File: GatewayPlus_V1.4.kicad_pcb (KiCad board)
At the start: 2 copper layers, 100 x 60 mm, 274 parts, among them IC1 MP1584EN, IC2 MP1584EN, J1 SWD_LOG, J10 USB_OTG, J11 USB_WIFI, J2 LTDC_LCD_FPC_40p, J3 Micro_SD_Card, J4 ESP Anten, J5 LoRa_Anten, J6 HR911105A, J7 RS485, J8 Conn_Jack-DC, J9 AudioJack, Q1 BC847, SW1 SW_Push, SW2 ESP_RESET, SW3 ESP_BOOT, U1 STM32F429IGTx, U10 USBLC6-2SC6, U11 USBLC6-2SC6, U2 IS42S16400J - HY57V641620E, U3 ESP32-C3, U4 W25Q32JVSS, U5 SX1278, U6 MASWSS0192, U7 LAN8720A, U8 MAX485E, U9 ES8388, Y1 25MHz, Y2 40MHz, Y3 32MHz, Y4 25MHz, Y5 32.768KHz

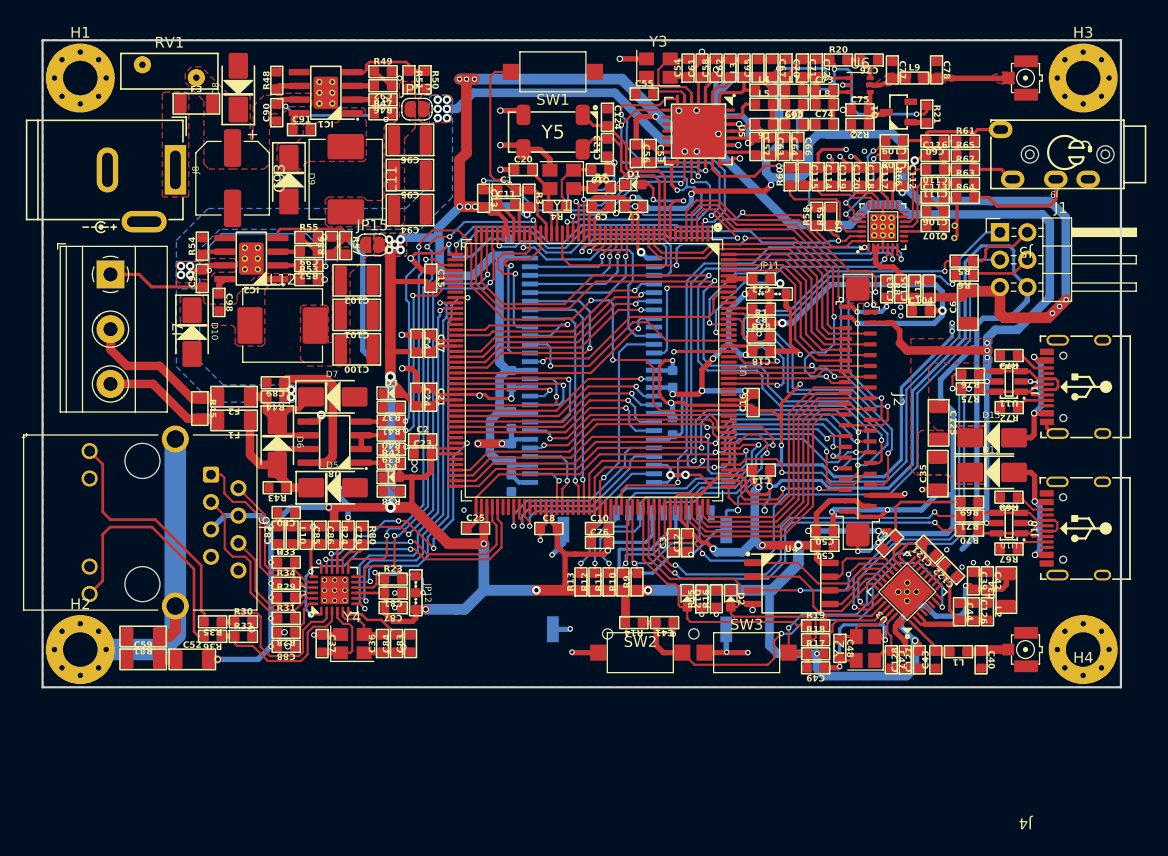
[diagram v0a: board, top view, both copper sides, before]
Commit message: Fix some bug.
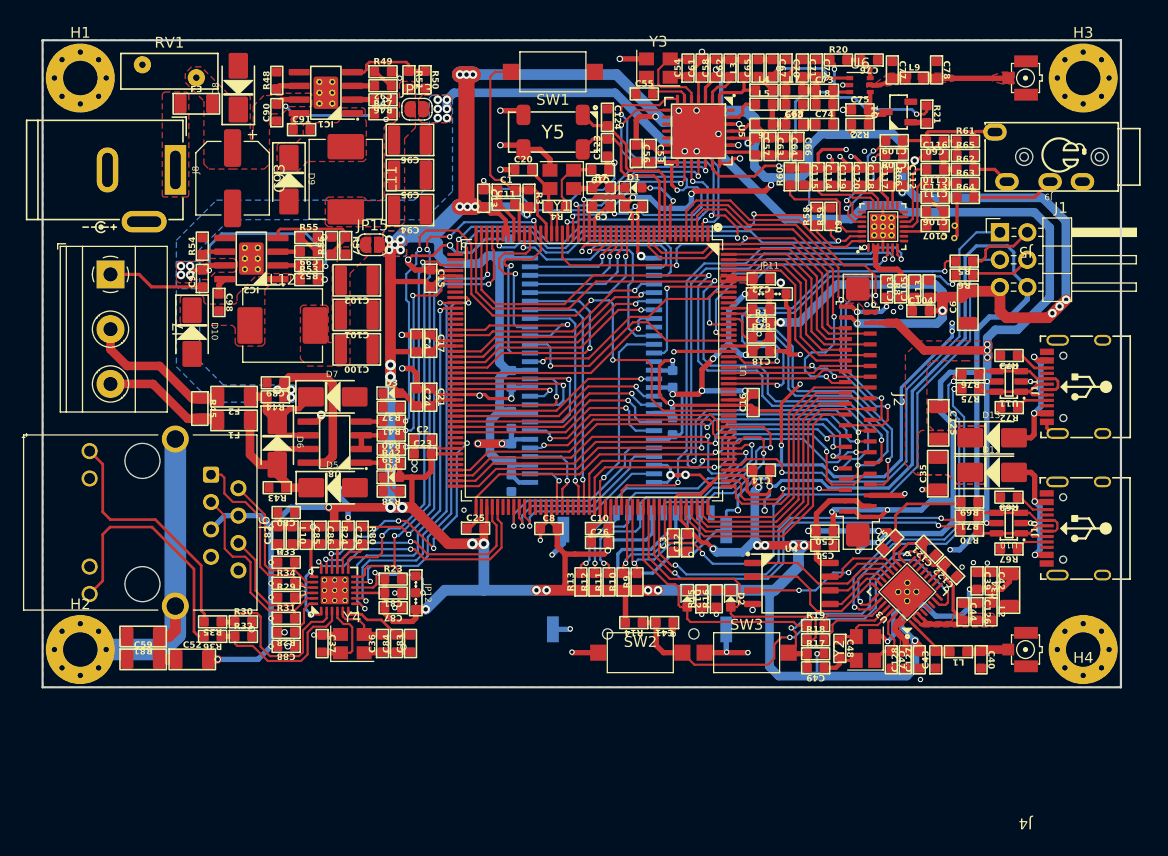
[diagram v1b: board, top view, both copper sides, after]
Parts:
- moved J9 0.58 mm to (136.6, 72.2)
- moved C42 0.34 mm to (131.3, 111.5)
- moved C39 0.33 mm to (130.0, 111.5)
- moved L2 0.33 mm to (131.3, 114.4)
- moved C126 0.32 mm to (130.0, 114.4)
- moved C44 0.32 mm to (128.7, 114.4)
- moved D1 0.29 mm to (98.2, 75.1)
- moved C34 0.29 mm to (133.0, 112.4)
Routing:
- net GND: track 556.0 -> 536.2 mm, vias 98 -> 97
- net +3.3V: track 648.5 -> 634.5 mm, vias 57 -> 64
- net STATUS LED: track 9.10 -> 6.56 mm
- net /AUDIO/ROUT: track 11.4 -> 8.99 mm
- net Net-(U5-RXTX/RF_MOD): track 33.8 -> 31.7 mm
- net /MCU/SDIO_D3: track 27.1 -> 25.8 mm
- net USART6_TX: track 32.8 -> 33.8 mm
- net WiFi_RST: track 40.4 -> 41.3 mm
- net /LTDC TFT LCD/LTDC_R1: track 60.0 -> 60.9 mm
- net /LTDC TFT LCD/LTDC_R0: track 61.4 -> 62.3 mm
- net USART6_RX: track 34.8 -> 35.7 mm
- net /MCU/SDIO_CLK: track 18.1 -> 17.3 mm
- net /MCU/SDRAM_NBL0: track 21.8 -> 21.1 mm
- net /WIFI ESP32/F_D2: track 14.8 -> 14.1 mm
- net /LORA/LoRa_IRQ: track 50.0 -> 49.3 mm
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- added copper zone on F.Cu, net Net-(U3-VDD3P3_CPU)
